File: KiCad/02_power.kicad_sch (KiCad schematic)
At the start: 38 parts, among them J201 Barrel_Jack_Switch_Pin3Ring, U201 AMS1117-3.3, U202 TLV62569DBV, U203 HT7533-1

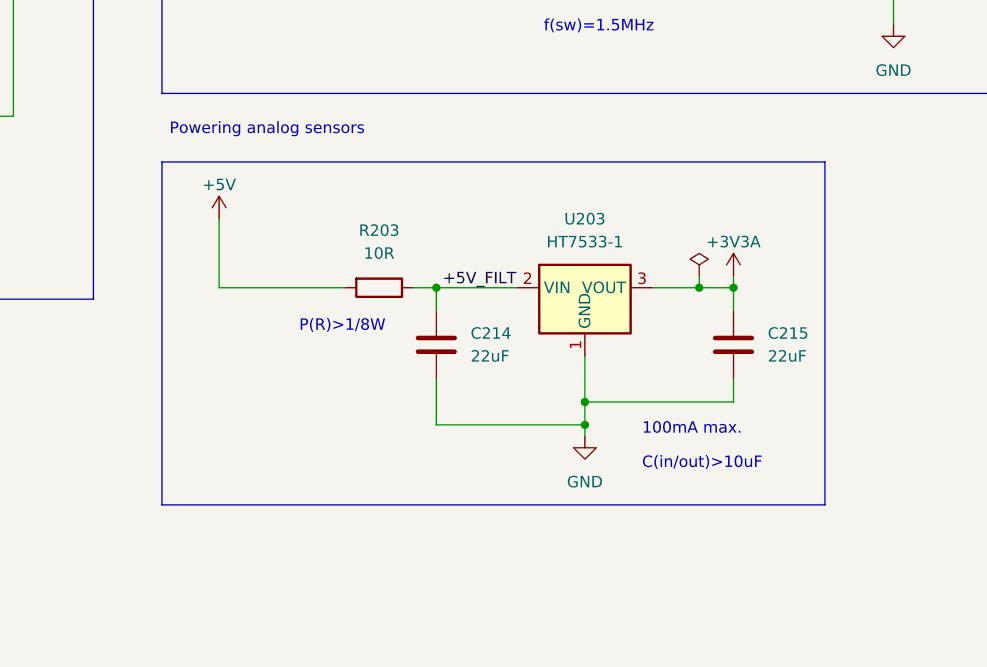
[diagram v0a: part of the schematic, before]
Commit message: First scheme version
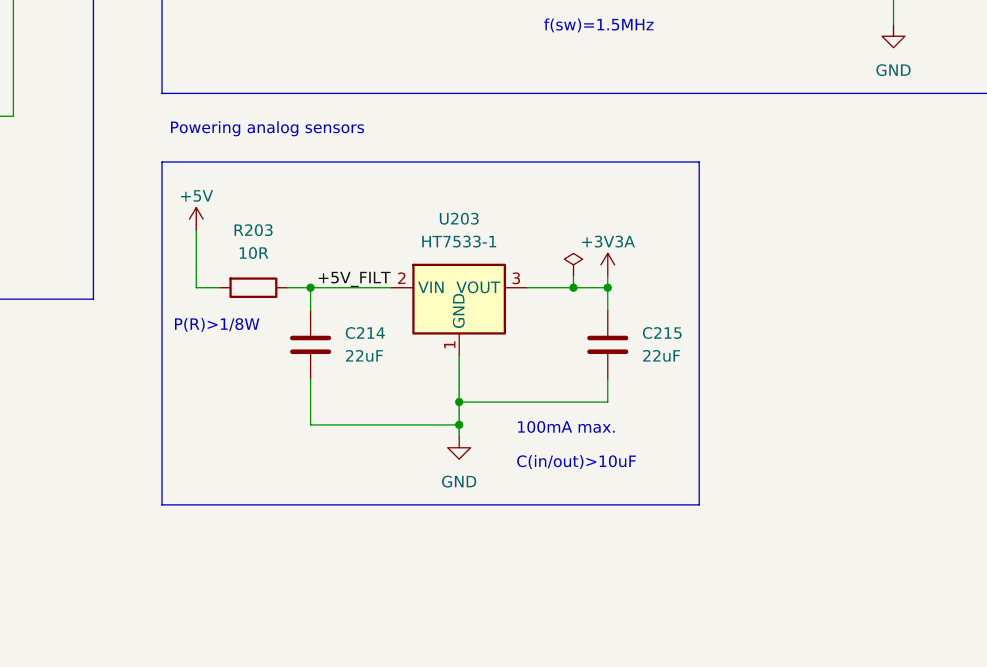
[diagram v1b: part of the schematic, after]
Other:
- moved on the sheet: C214, C215, R203, U203
